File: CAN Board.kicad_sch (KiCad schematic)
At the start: 37 parts, among them J1 Conn_02x07_Odd_Even, J3 USB_C_Receptacle_USB2.0_16P, J4 Conn_01x02, J5 Conn_01x02, J6 Conn_01x02, J7 Conn_01x02, J8 Conn_01x02, J9 Conn_01x02, SW1 SW_Push, SW2 SW_Push, U1 RP2040, U2 W25Q128JVS, U3 MIC5504-3.3YM5, Y1 Crystal_GND24

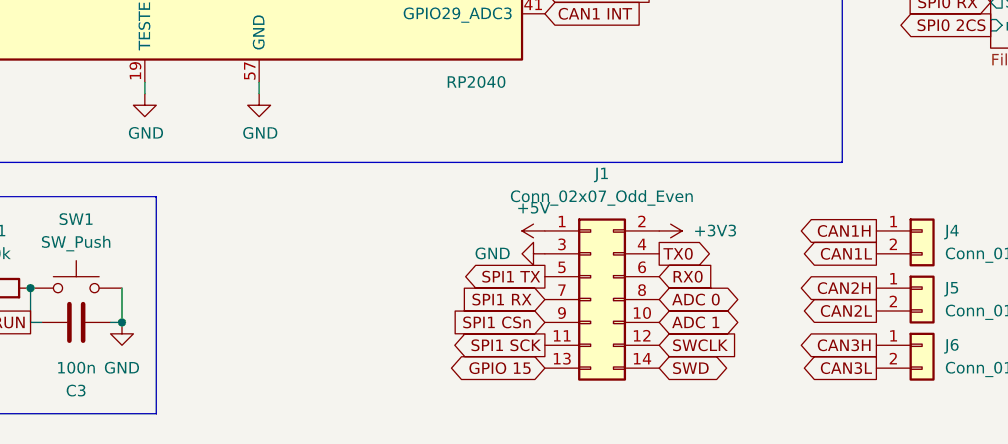
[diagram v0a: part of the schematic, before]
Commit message: it has no errors :)
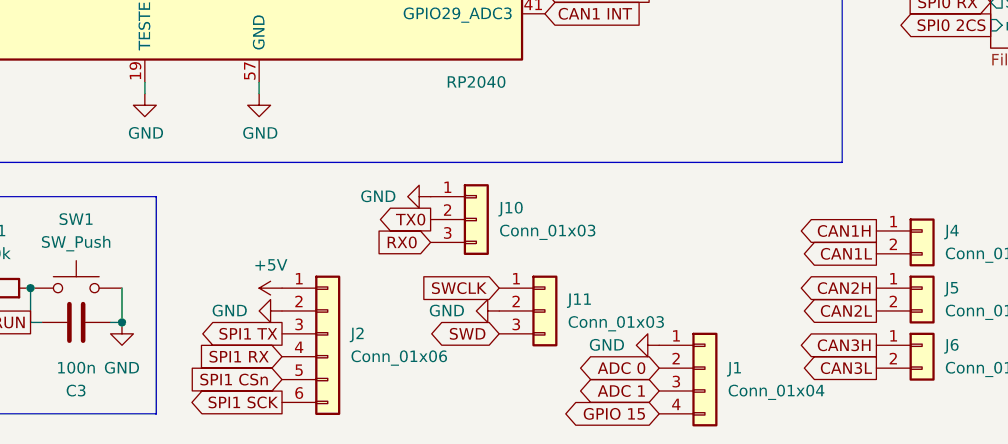
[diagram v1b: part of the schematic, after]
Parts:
- removed J1: Conn_02x07_Odd_Even, Connector_PinHeader_2.54mm:PinHeader_2x07_P2.54mm_Vertical, symbol Connector_Generic:Conn_02x07_Odd_Even
- added J1: Conn_01x04, Connector_Molex:Molex_PicoBlade_53047-0410_1x04_P1.25mm_Vertical, symbol Connector_Generic:Conn_01x04
- added J10, J11: Conn_01x03, Connector_Molex:Molex_PicoBlade_53047-0310_1x03_P1.25mm_Vertical, symbol Connector_Generic:Conn_01x03
- added J2: Conn_01x06, Connector_Molex:Molex_PicoBlade_53047-0610_1x06_P1.25mm_Vertical, symbol Connector_Generic:Conn_01x06
- J3: footprint Connector_USB:USB_C_Receptacle_GCT_USB4085 -> Connector_USB:USB_C_Receptacle_G-Switch_GT-USB-7010ASV
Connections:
- net +5V: now also J2.1 (Pin_1)
- net ADC 0: now also J1.2 (Pin_2)
- net ADC 1: now also J1.3 (Pin_3)
- net GND: now also J1.1 (Pin_1), J10.1 (Pin_1), J11.2 (Pin_2), J2.2 (Pin_2)
- net GPIO 15: now also J1.4 (Pin_4)
- net RX0: now also J10.3 (Pin_3)
- net SPI1 CSn: now also J2.5 (Pin_5)
- net SPI1 RX: now also J2.4 (Pin_4)
- net SPI1 SCK: now also J2.6 (Pin_6)
- net SPI1 TX: now also J2.3 (Pin_3)
- net SWCLK: now also J11.1 (Pin_1)
- net SWD: now also J11.3 (Pin_3)
- net TX0: now also J10.2 (Pin_2)

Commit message: cleaning up and minor updates
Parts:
- J3: footprint Connector_USB:USB_C_Receptacle_G-Switch_GT-USB-7010ASV -> Connector_USB:USB_C_Receptacle_GCT_USB4105-xx-A_16P_TopMnt_Horizontal
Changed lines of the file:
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@@
 			)
 		)
-		(property "Footprint" "Connector_USB:USB_C_Receptacle_G-Switch_GT-USB-7010ASV"
+		(property "Footprint" "Connector_USB:USB_C_Receptacle_GCT_USB4105-xx-A_16P_TopMnt_Horizontal"
 			(at 255.27 40.64 0)
 			(effects

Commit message: added mounting holes
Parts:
- J4, J5, J6, J7, J8, J9: footprint Connector_PinHeader_2.54mm:PinHeader_1x02_P2.54mm_Vertical -> Connector_PinSocket_2.54mm:PinSocket_1x02_P2.54mm_Vertical
- R6: now left out of the parts list
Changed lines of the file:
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@@
 			)
 		)
-		(property "Footprint" "Connector_PinHeader_2.54mm:PinHeader_1x02_P2.54mm_Vertical"
+		(property "Footprint" "Connector_PinSocket_2.54mm:PinSocket_1x02_P2.54mm_Vertical"
 			(at 157.48 176.53 0)
 			(effects
@@
 			)
 		)
-		(property "Footprint" "Connector_PinHeader_2.54mm:PinHeader_1x02_P2.54mm_Vertical"
+		(property "Footprint" "Connector_PinSocket_2.54mm:PinSocket_1x02_P2.54mm_Vertical"
 			(at 157.48 189.23 0)
 			(effects
@@
 			)
 		)
-		(property "Footprint" "Connector_PinHeader_2.54mm:PinHeader_1x02_P2.54mm_Vertical"
+		(property "Footprint" "Connector_PinSocket_2.54mm:PinSocket_1x02_P2.54mm_Vertical"
 			(at 157.48 182.88 0)
 			(effects
@@
 			)
 		)
-		(property "Footprint" "Connector_PinHeader_2.54mm:PinHeader_1x02_P2.54mm_Vertical"
+		(property "Footprint" "Connector_PinSocket_2.54mm:PinSocket_1x02_P2.54mm_Vertical"
 			(at 132.08 182.88 0)
 			(effects
@@
 			)
 		)
-		(property "Footprint" "Connector_PinHeader_2.54mm:PinHeader_1x02_P2.54mm_Vertical"
+		(property "Footprint" "Connector_PinSocket_2.54mm:PinSocket_1x02_P2.54mm_Vertical"
 			(at 132.08 176.53 0)
 			(effects
@@
 			)
 		)
-		(property "Footprint" "Connector_PinHeader_2.54mm:PinHeader_1x02_P2.54mm_Vertical"
+		(property "Footprint" "Connector_PinSocket_2.54mm:PinSocket_1x02_P2.54mm_Vertical"
 			(at 132.08 189.23 0)
 			(effects
@@
 		(unit 1)
 		(exclude_from_sim no)
-		(in_bom yes)
+		(in_bom no)
 		(on_board yes)
 		(dnp yes)
